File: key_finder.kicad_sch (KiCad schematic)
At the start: 27 parts, among them J1 Conn_ARM_JTAG_SWD_10, SW1 SW_Push, SW2 SW_Push, U1 NRF52832, X1 32MHz, X2 32.768kHz

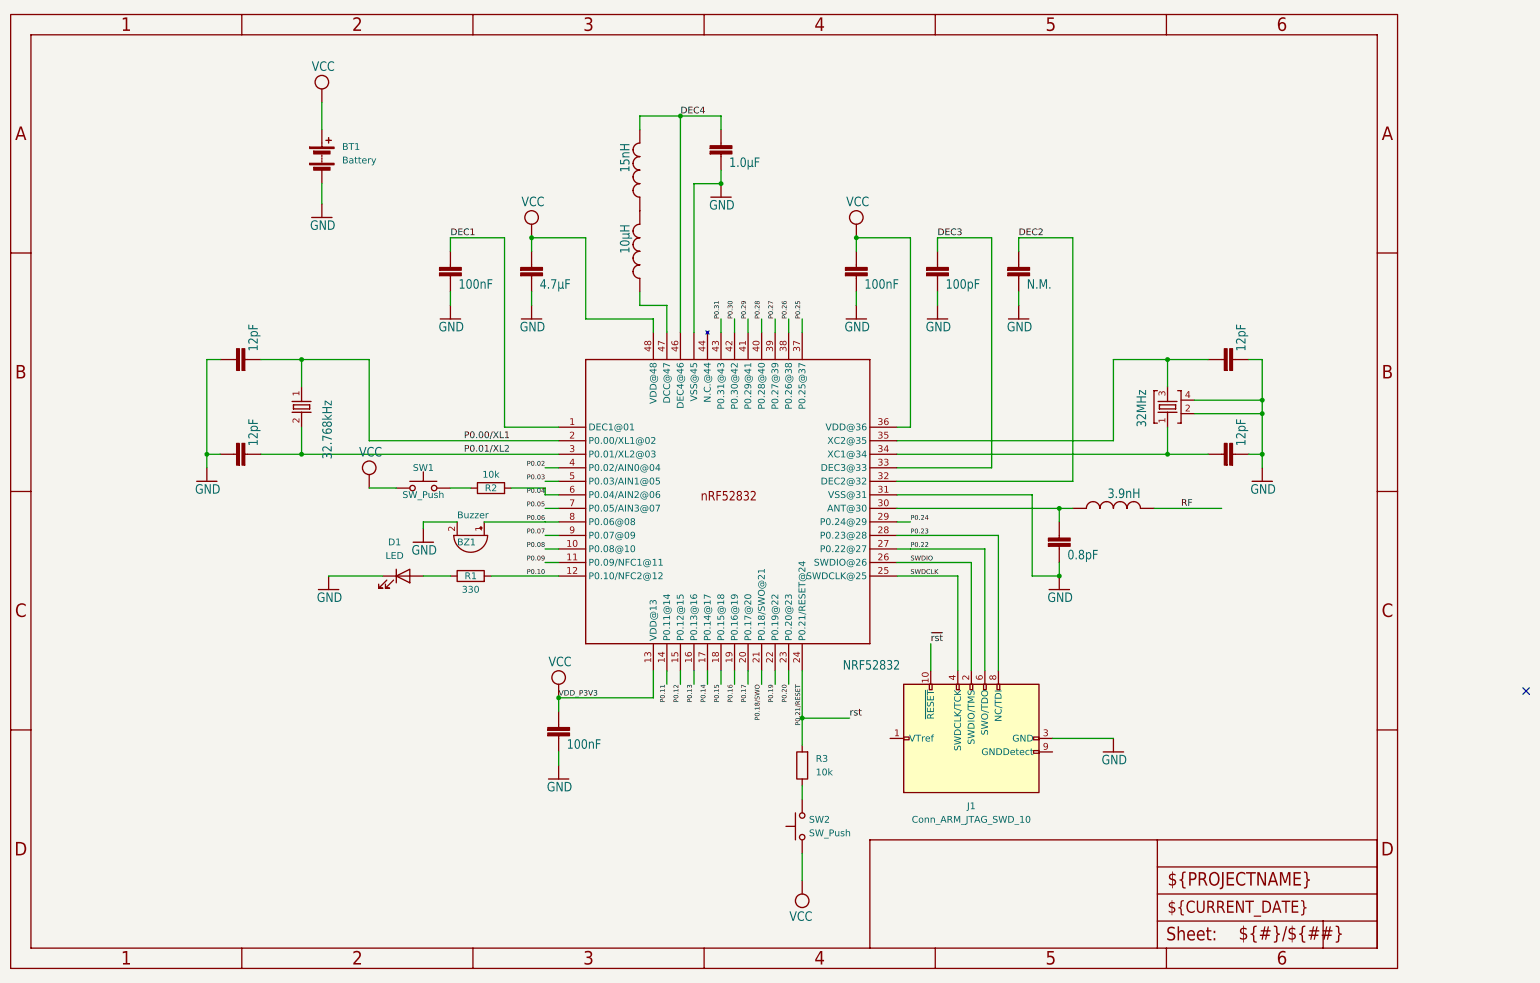
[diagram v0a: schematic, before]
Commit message: sceance 2
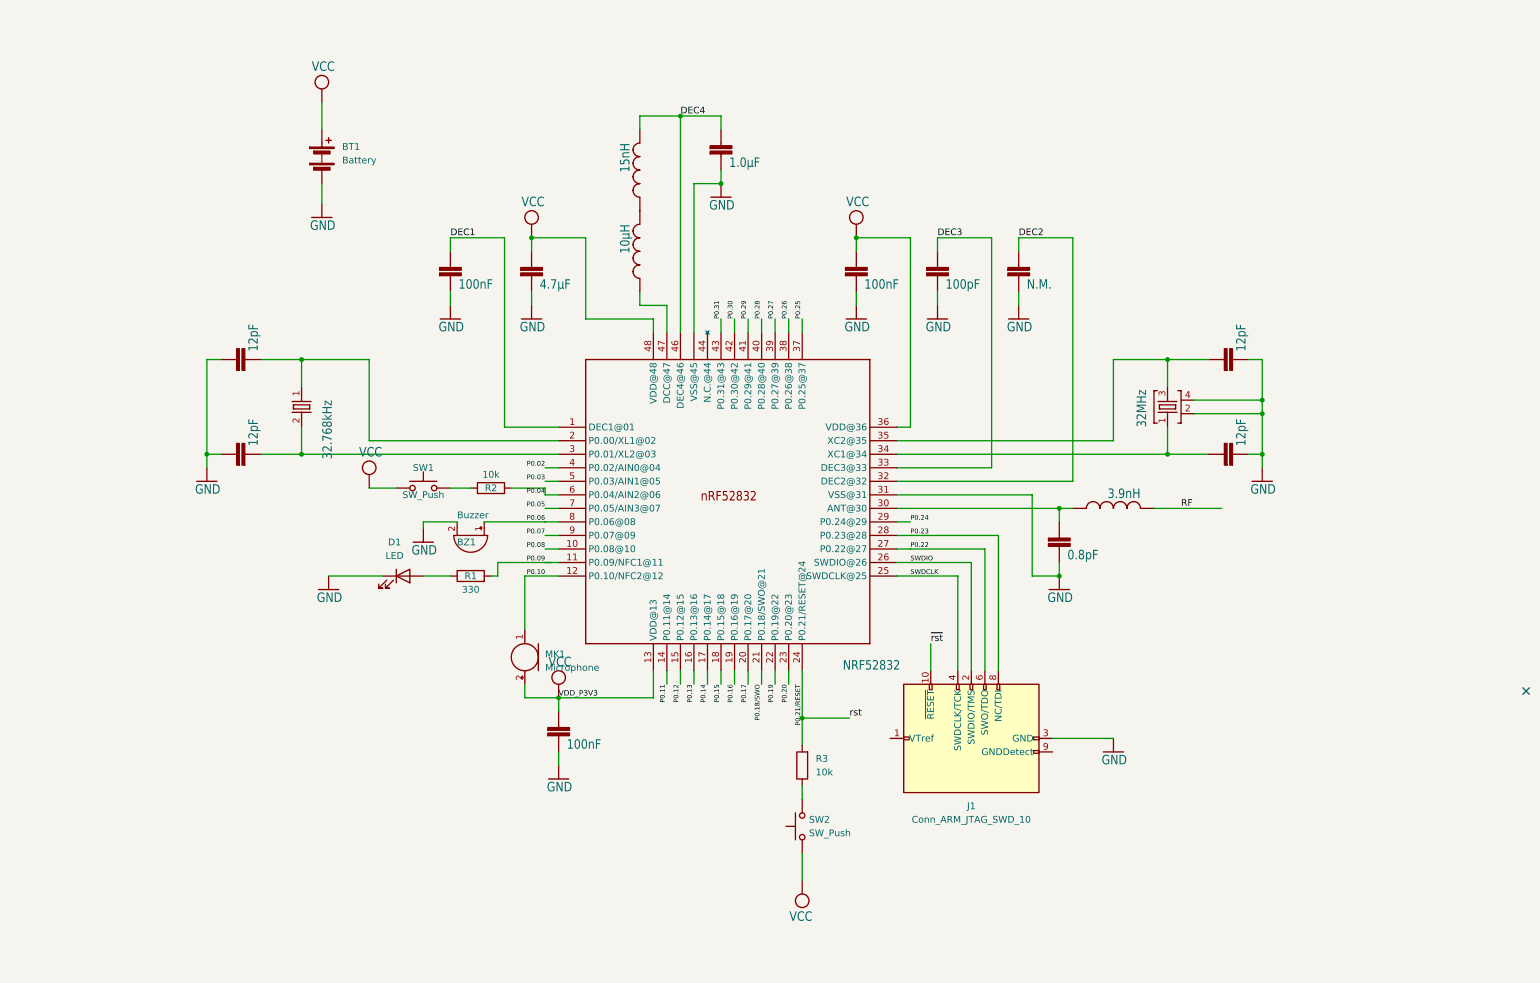
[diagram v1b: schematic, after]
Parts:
- added MK1: Microphone, Sensor_Audio:CUI_CMC-4013-SMT, symbol Device:Microphone
- BT1: footprint Battery:BatteryHolder_Keystone_1057_1x2032 -> Battery:BatteryHolder_Keystone_1060_1x2032; PRM 36-1057-ND -> 36-1060-ND
- SW1: footprint Button_Switch_THT:SW_PUSH_6mm_H7.3mm -> Button_Switch_SMD:SW_Push_1P1T_NO_CK_KMR2; PRM TS04-66-50-BK-160-SMT -> KMR223GLFG
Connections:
- net P0.09: now also R1.2
- net P0.10: now also MK1.1 (-); no longer R1.2
- net VCC: now also MK1.2 (+)
- net P0.00/XL1: no longer names the net of C11.2, U1.2 (P0.00/XL1@02), X2.1
- net P0.01/XL2: no longer names the net of C12.2, U1.3 (P0.01/XL2@03), X2.2
